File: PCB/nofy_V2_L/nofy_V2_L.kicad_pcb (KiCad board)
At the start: 2 copper layers, 99.7 x 78.9 mm, 70 parts, among them J18 PIn1x4, SW10 SW_PUSH, SW11 SW_PUSH, SW13 SW_PUSH, SW14 SW_PUSH, SW15 SW_PUSH, SW17 SW_PUSH, SW18 SW_PUSH, SW19 SW_PUSH, SW20 SW_PUSH, SW21 SW_PUSH, SW22 SW_PUSH, SW23 SW_PUSH, SW24 SW_PUSH, SW25 SW_PUSH, SW26 SW_PUSH, SW27 SW_PUSH, SW28 SW_PUSH, SW29 SW_PUSH, SW3 RotaryEncoder, SW30 SW_PUSH, SW31 SW_PUSH, SW5 SW_PUSH, SW6 SW_PUSH, SW7 SW_PUSH, SW9 SW_PUSH

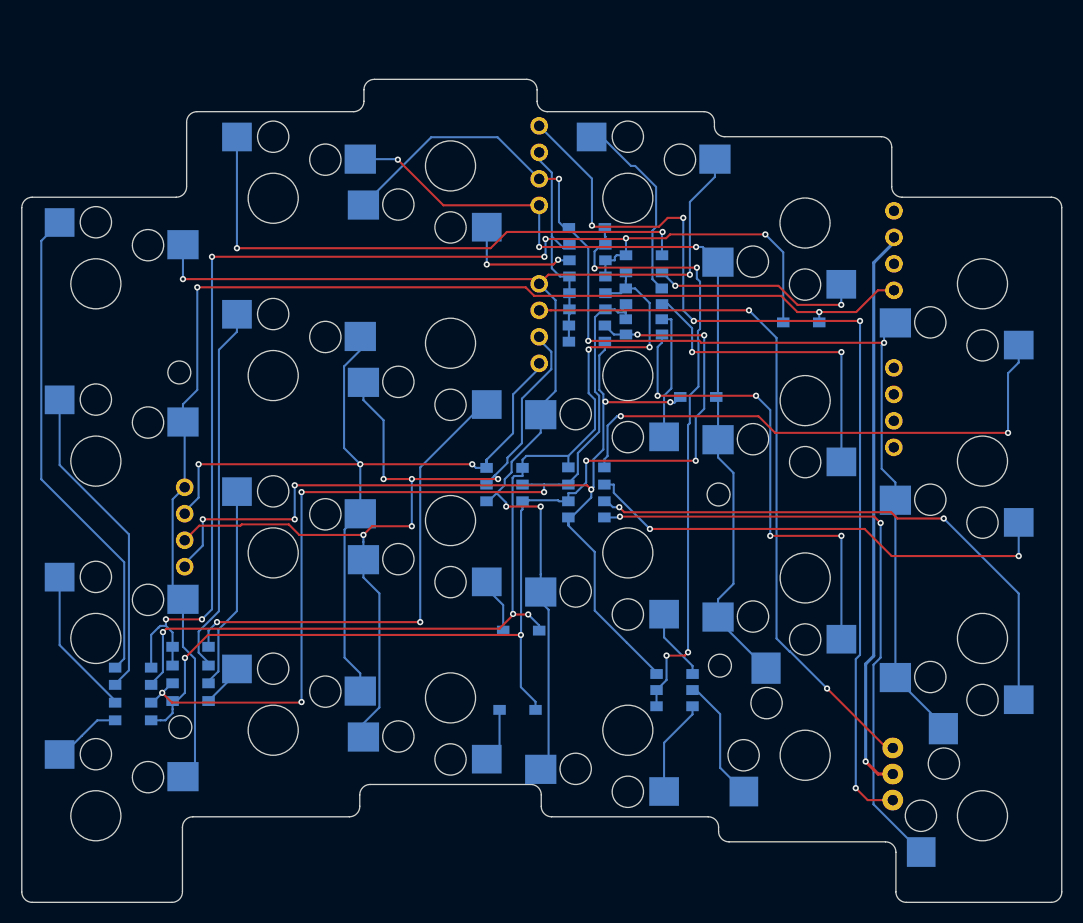
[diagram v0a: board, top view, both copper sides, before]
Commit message: pcb
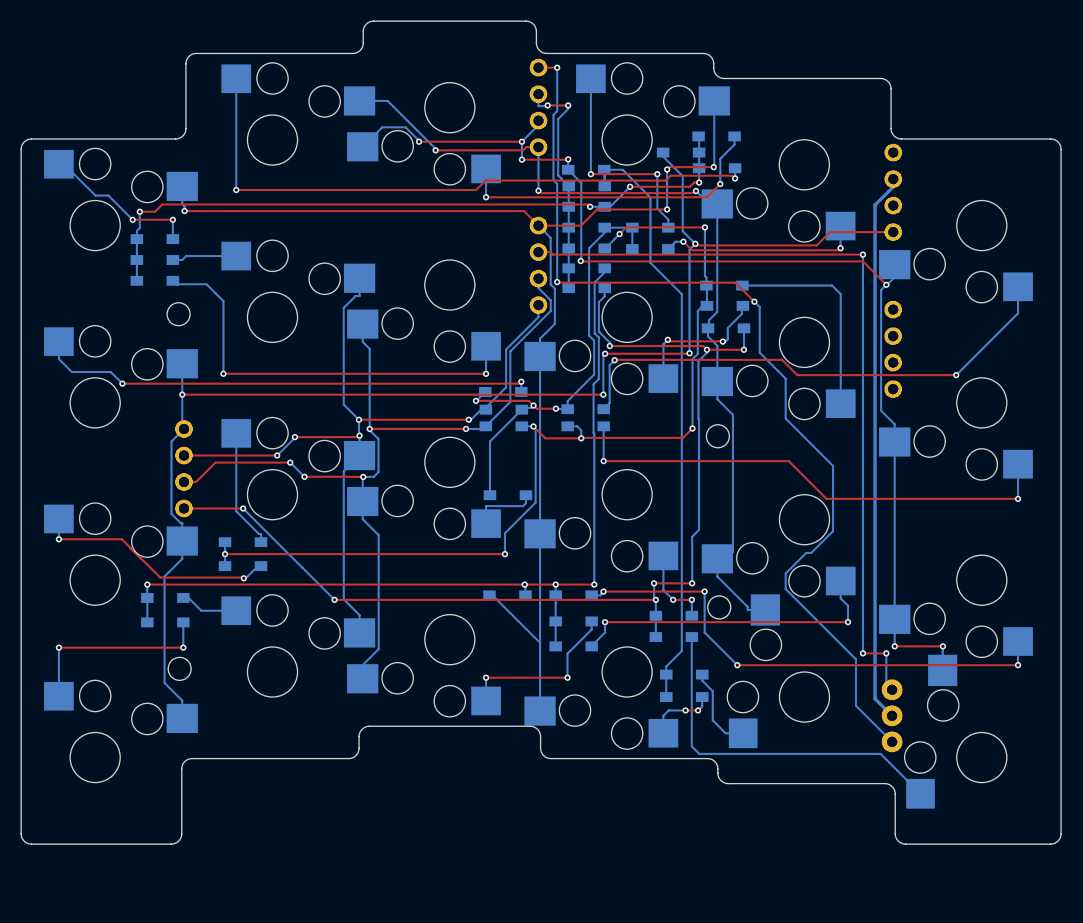
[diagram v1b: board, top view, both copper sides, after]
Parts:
- D1, D10, D11, D13, D14, D15, D16, D17, D18, D19, D2, D20, D21, D22, D23, D24, D25, D26, D27, D3, D5, D6, D7, D9, DI1, DI2, DI3, DI4, DI5, DI6, DS1, DS2, DS3, DS4, DS5, DS6: moved to F.Cu
- moved D13 41.2 mm to (27.2, 42.4), turned to 0 degrees
- moved D1 41.0 mm to (60.6, 57.0), turned to 0 degrees
- moved D5 39.0 mm to (27.2, 44.4)
- moved D9 35.2 mm to (27.2, 46.4)
- moved D21 30.7 mm to (67.4, 81.4)
- moved DS1 23.6 mm to (77.7, 34.0), turned to 0 degrees
- moved D10 14.7 mm to (61.1, 66.9), turned to 0 degrees
- moved D6 14.4 mm to (35.7, 71.4)
- moved D27 14.2 mm to (77.0, 80.5)
- moved D2 14.0 mm to (35.7, 73.7), turned to 0 degrees
- moved D23 13.7 mm to (81.1, 32.5), turned to 0 degrees
- moved D18 10.9 mm to (81.1, 35.5)
- moved D7 10.2 mm to (28.2, 76.8)
- moved D3 9.70 mm to (28.2, 79.1), turned to 0 degrees
- moved D26 9.10 mm to (67.4, 76.5)
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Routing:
- net Net-(D13-K): track 117.8 -> 66.1 mm, vias 7 -> 4
- net Net-(D1-K): track 92.8 -> 45.3 mm, vias 5 -> 3
- net Net-(D13-A): track 47.1 -> 15.0 mm, vias 0 -> 2
- net Net-(D5-A): track 35.6 -> 6.23 mm
- net Net-(D27-A): track 60.5 -> 34.3 mm, vias 2 -> 0
- net Net-(D11-K): track 104.7 -> 84.6 mm, vias 6 -> 4
- net Net-(D23-A): track 11.7 -> 30.8 mm
- net Net-(D1-A): track 30.6 -> 48.0 mm, vias 0 -> 2
- net Net-(D21-A): track 46.2 -> 30.4 mm, vias 4 -> 2
- net Net-(D3-A): track 6.68 -> 19.0 mm, vias 0 -> 2
- net Net-(D11-A): track 5.23 -> 16.4 mm, vias 0 -> 2
- net Net-(D20-A): track 31.0 -> 20.3 mm, vias 2 -> 0
- net Net-(D16-K): track 91.5 -> 102.1 mm, vias 6 -> 8
- net Pin0: track 119.0 -> 129.3 mm, vias 2 -> 5
- net Net-(D2-A): track 14.2 -> 23.4 mm, vias 0 -> 2
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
